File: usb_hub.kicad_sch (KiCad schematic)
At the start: 17 parts, among them U4 RTS5411-GRT, Y1 24MHz

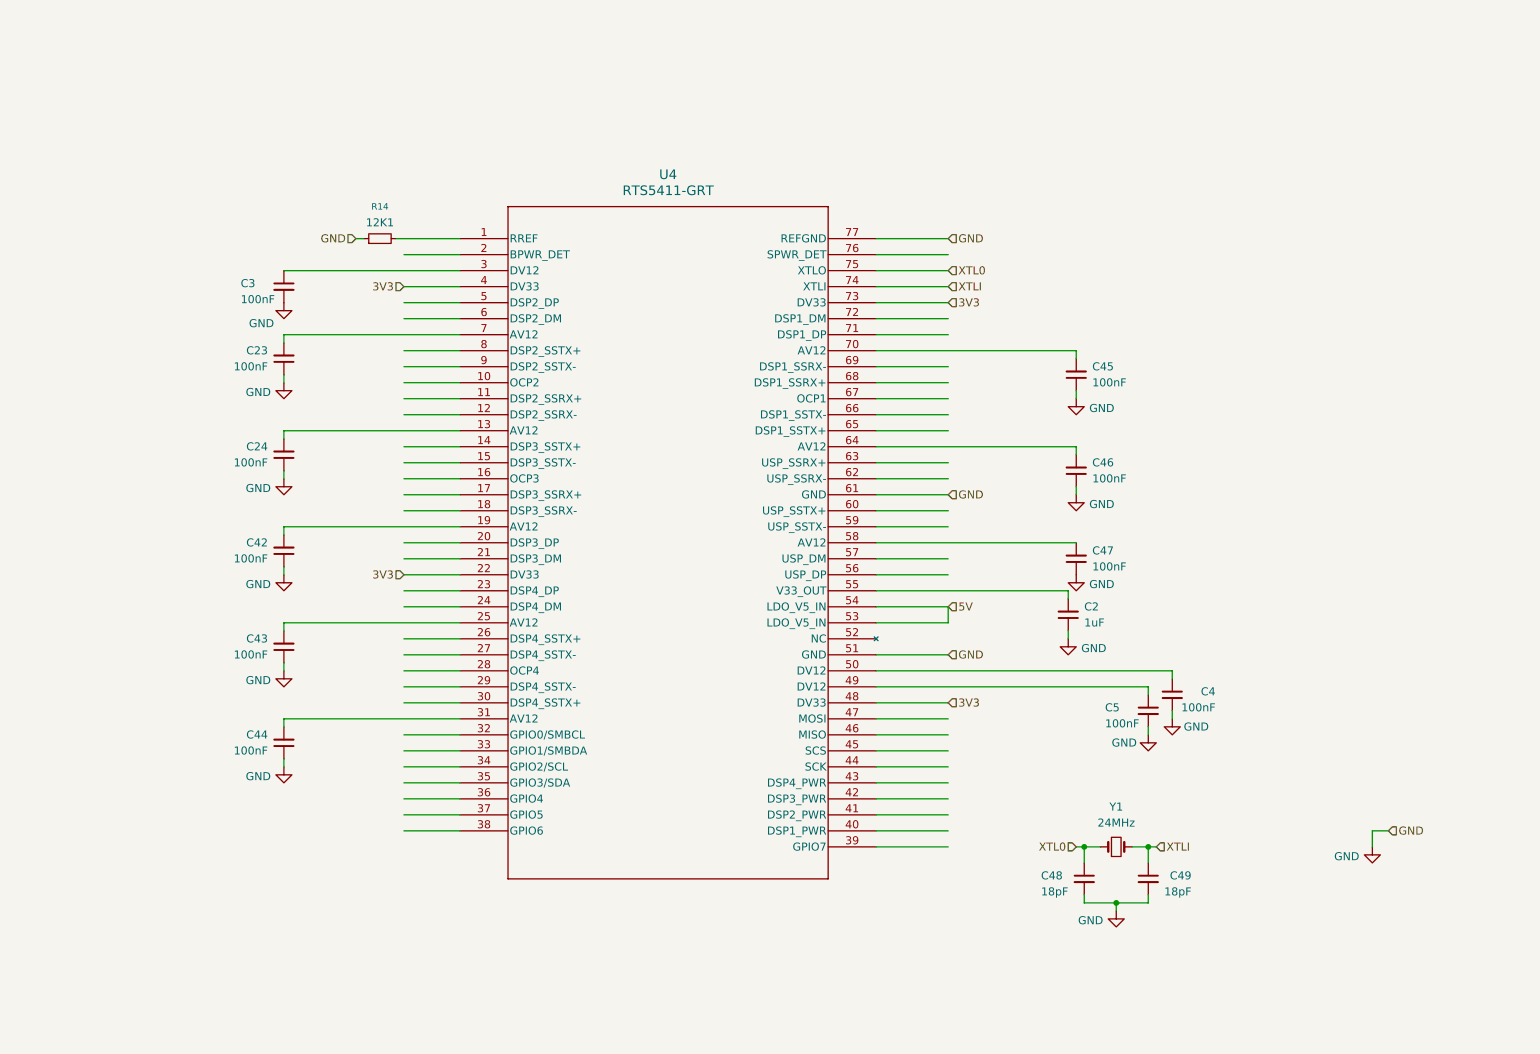
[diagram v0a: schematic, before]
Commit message: Add files via upload
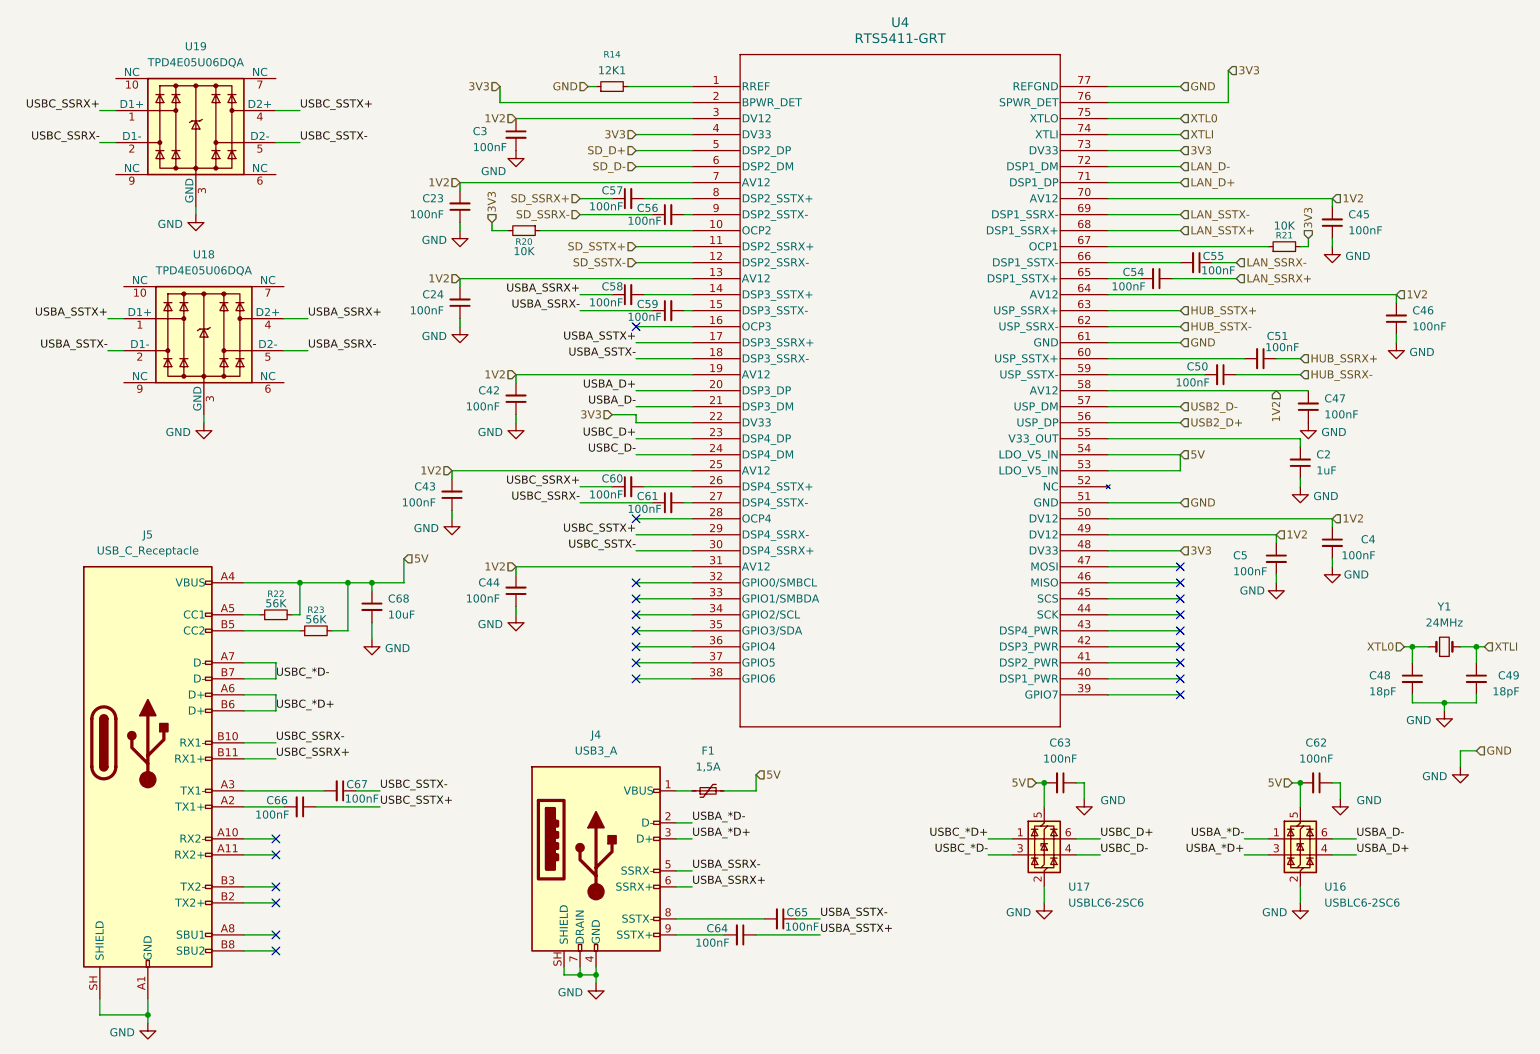
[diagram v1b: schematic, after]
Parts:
- added C50, C51, C54, C55, C56, C57, C58, C59, C60, C61, C62, C63, C64, C65, C66, C67: 100nF, symbol Device:C_Small
- added C68: 10uF, symbol Device:C_Small
- added F1: 1,5A, symbol Device:Polyfuse_Small
- added J4: USB3_A, symbol Connector:USB3_A
- added J5: USB_C_Receptacle, Connector_USB:USB_C_Receptacle_Molex_105450-0101, symbol Connector:USB_C_Receptacle
- added R20, R21: 10K, symbol Device:R_Small
- added R22, R23: 56K, symbol Device:R_Small
- added U16, U17: USBLC6-2SC6, Package_TO_SOT_SMD:SOT-23-6, symbol Power_Protection:USBLC6-2SC6
- added U18, U19: TPD4E05U06DQA, Package_SON:USON-10_2.5x1.0mm_P0.5mm, symbol Power_Protection:TPD4E05U06DQA
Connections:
- net 3V3: now also U4.2 (BPWR_DET), U4.76 (SPWR_DET), R20.2, R21.2
- net 5V: now also C62.2, C63.2, C68.1, F1.2, J5.A4 (VBUS), J5.A9 (VBUS), J5.B4 (VBUS), J5.B9 (VBUS), R22.2, R23.2, U16.5 (VBUS), U17.5 (VBUS)
- net GND: now also C62.1, C63.1, C68.2, J4.4 (GND), J4.7 (DRAIN), J4.SH (SHIELD), J5.A1 (GND), J5.A12 (GND), J5.B1 (GND), J5.B12 (GND), J5.SH (SHIELD), U16.2 (GND), U17.2 (GND), U18.3 (GND), U18.8 (GND), U19.3 (GND), U19.8 (GND)
- net 1V2: now reaches C4.1, U4.50 (DV12)
- net 1V2: now also C23.2, C24.2, C3.1, C42.2, C43.2, C44.2, C45.2, C46.2, C47.2, C5.1, U4.13 (AV12), U4.19 (AV12), U4.25 (AV12), U4.3 (DV12), U4.31 (AV12), U4.49 (DV12), U4.58 (AV12), U4.64 (AV12), U4.7 (AV12), U4.70 (AV12)
- net at U4.10 (OCP2): now also R20.1
- net SD_SSTX+: now reaches U4.11 (DSP2_SSRX+)
- net SD_SSTX-: now reaches U4.12 (DSP2_SSRX-)
- net at U4.14 (DSP3_SSTX+): now also C58.2
- net at U4.15 (DSP3_SSTX-): now also C59.2
- net USBA_SSTX+: now reaches U4.17 (DSP3_SSRX+)
- net USBA_SSTX+: now also C64.1, U18.1 (D1+)
- net USBA_SSTX-: now reaches U4.18 (DSP3_SSRX-)
- net USBA_SSTX-: now also C65.1, U18.2 (D1-)
- net USBA_D+: now reaches U4.20 (DSP3_DP)
- net USBA_D+: now also U16.4 (I/O2)
- net USBA_D-: now reaches U4.21 (DSP3_DM)
- net USBA_D-: now also U16.6 (I/O1)
- net USBC_D+: now reaches U4.23 (DSP4_DP)
- net USBC_D+: now also U17.6 (I/O1)
- net USBC_D-: now reaches U4.24 (DSP4_DM)
- net USBC_D-: now also U17.4 (I/O2)
- net at U4.26 (DSP4_SSTX+): now also C60.2
- net at U4.27 (DSP4_SSTX-): now also C61.2
- net USBC_SSTX+: now reaches U4.29 (DSP4_SSRX-)
- net USBC_SSTX+: now also C66.1, U19.4 (D2+)
- net USBC_SSTX-: now reaches U4.30 (DSP4_SSRX+)
- net USBC_SSTX-: now also C67.1, U19.5 (D2-)
- net SD_D+: now reaches U4.5 (DSP2_DP)
- net USB2_D+: now reaches U4.56 (USP_DP)
- net USB2_D-: now reaches U4.57 (USP_DM)
- net at U4.59 (USP_SSTX-): now also C50.2
- net SD_D-: now reaches U4.6 (DSP2_DM)
- net at U4.60 (USP_SSTX+): now also C51.2
- net HUB_SSTX-: now reaches U4.62 (USP_SSRX-)
- net HUB_SSTX+: now reaches U4.63 (USP_SSRX+)
- net at U4.65 (DSP1_SSTX+): now also C54.2
- net at U4.66 (DSP1_SSTX-): now also C55.2
- net at U4.67 (OCP1): now also R21.1
- net LAN_SSTX+: now reaches U4.68 (DSP1_SSRX+)
- net LAN_SSTX-: now reaches U4.69 (DSP1_SSRX-)
- net LAN_D+: now reaches U4.71 (DSP1_DP)
- net LAN_D-: now reaches U4.72 (DSP1_DM)
- net at U4.8 (DSP2_SSTX+): now also C57.2
- net at U4.9 (DSP2_SSTX-): now also C56.2
- new net: C65.2, J4.8 (SSTX-)
- new net: J5.A5 (CC1), R22.1
- new net: C66.2, J5.A2 (TX1+)
- new net: C67.2, J5.A3 (TX1-)
- new net: J5.B5 (CC2), R23.1
- new net: C64.2, J4.9 (SSTX+)
- new net: F1.1, J4.1 (VBUS)
- new net HUB_SSRX+: C51.1
- new net HUB_SSRX-: C50.1
- new net LAN_SSRX+: C54.1
- new net LAN_SSRX-: C55.1
- new net SD_SSRX+: C57.1
- new net SD_SSRX-: C56.1
- new net USBA_*D+: J4.3 (D+), U16.3 (I/O2)
- new net USBA_*D-: J4.2 (D-), U16.1 (I/O1)
- new net USBA_SSRX+: C58.1, J4.6 (SSRX+), U18.4 (D2+)
- new net USBA_SSRX-: C59.1, J4.5 (SSRX-), U18.5 (D2-)
- new net USBC_*D+: J5.A6 (D+), J5.B6 (D+), U17.1 (I/O1)
- new net USBC_*D-: J5.A7 (D-), J5.B7 (D-), U17.3 (I/O2)
- new net USBC_SSRX+: C60.1, J5.B11 (RX1+), U19.1 (D1+)
- new net USBC_SSRX-: C61.1, J5.B10 (RX1-), U19.2 (D1-)
- no-connect marks 0 -> 24
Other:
- moved on the sheet: C2, C23, C24, C3, C4, C42, C43, C44, C45, C46, C47, C48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
